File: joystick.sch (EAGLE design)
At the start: 2 parts, among them U1 JOYSTICKPTH

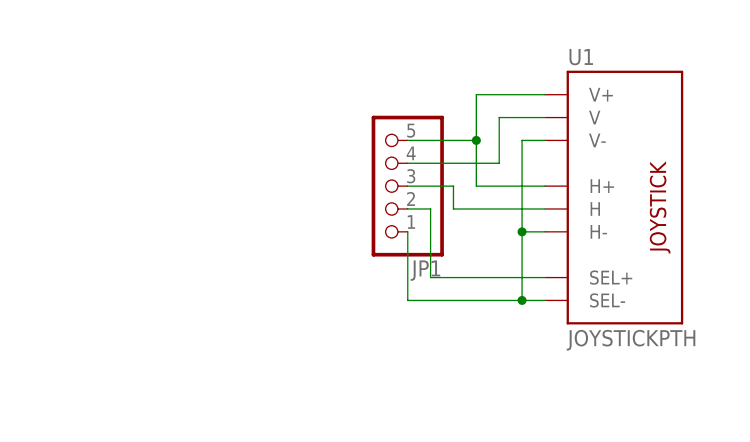
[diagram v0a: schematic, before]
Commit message: Initial upload of fork
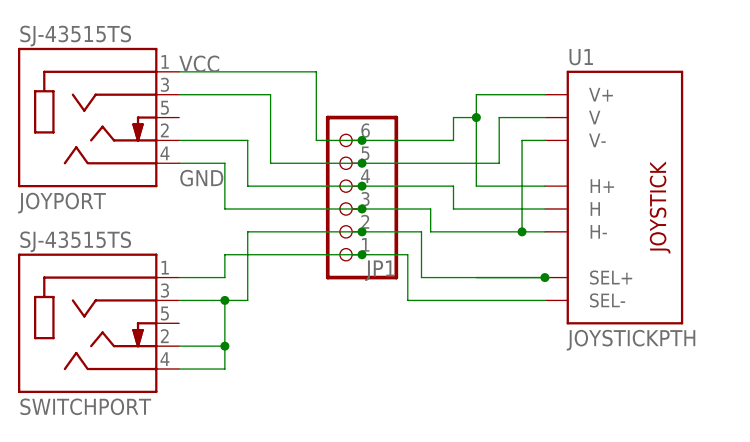
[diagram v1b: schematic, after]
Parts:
- added JOYPORT, SWITCHPORT: SJ-43515TS, ATMakers:SJ-43515TS
- JP1: device pinhead:PINHD-1X5 -> adafruit:PINHD-1X6B
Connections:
- removed net N$1: JP1.5, U1.H+, U1.V+
- new net GND: JOYPORT.RING2, JP1.3, U1.H-, U1.V-
- new net VCC: JOYPORT.SLEEVE, JP1.6, U1.H+, U1.V+
- net N$2: now also JP1.2, SWITCHPORT.RING1, SWITCHPORT.RING2, SWITCHPORT.TIP, U1.SEL+; no longer JP1.1, U1.H-, U1.SEL-, U1.V-
- net N$3: now also JOYPORT.RING1, JP1.5; no longer JP1.4
- net N$4: now also JOYPORT.TIP, JP1.4; no longer JP1.3
- net N$5: now also JP1.1, SWITCHPORT.SLEEVE, U1.SEL-; no longer JP1.2, U1.SEL+
